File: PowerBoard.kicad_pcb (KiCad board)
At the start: 2 copper layers, 131 x 131 mm, 106 parts, among them IC1 LT1910ES8#PBF, IC2 LT1910ES8#PBF, IC3 LT1910ES8#PBF, IC4 LT1910ES8#PBF, J1 XT90, J10 DEAN_T, J11 DEAN_T, J12 DEAN_T, J13 DEAN_T, J14 DEAN_T, J15 DEAN_T, J16 XT60, J17 XT60, J18 XT60, J19 XT60, J2 DEAN_T, J20 XT60, J21 XT60, J22 XT30, J23 XT30, J24 XT30, J25 XT30, J26 XT30, J27 XT30, J28 XT90, J29 XT30, J3 XT60, J30 XT30, J31 XT30, J32 Conn_01x02, J4 XT30, J5 XT90, J6 XT90, J7 XT90, J8 XT90, J9 XT90, Q1 IRFS7437TRLPBF, Q2 IRFS7437TRLPBF, Q3 IRFS7437TRLPBF, Q5 IRFS7530-7PPBF, U1 Pico, U2 LM317_TO-220

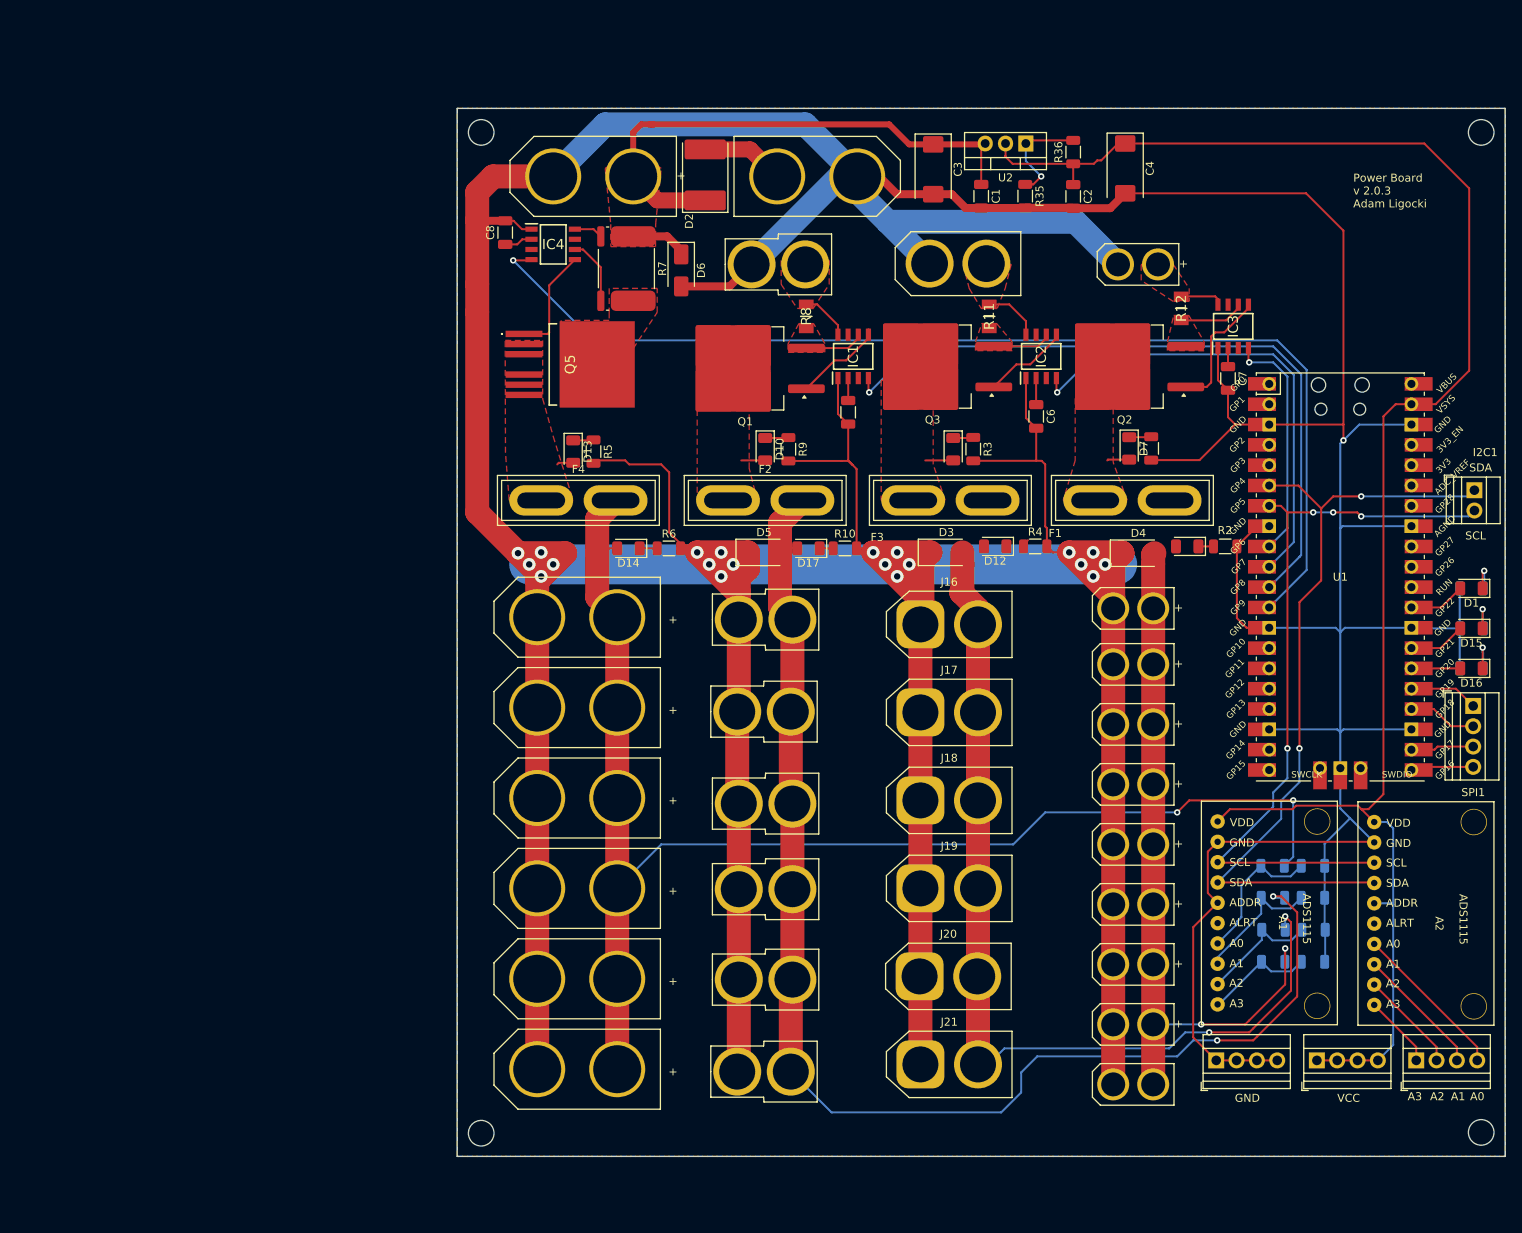
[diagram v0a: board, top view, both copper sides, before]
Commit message: Finish the design
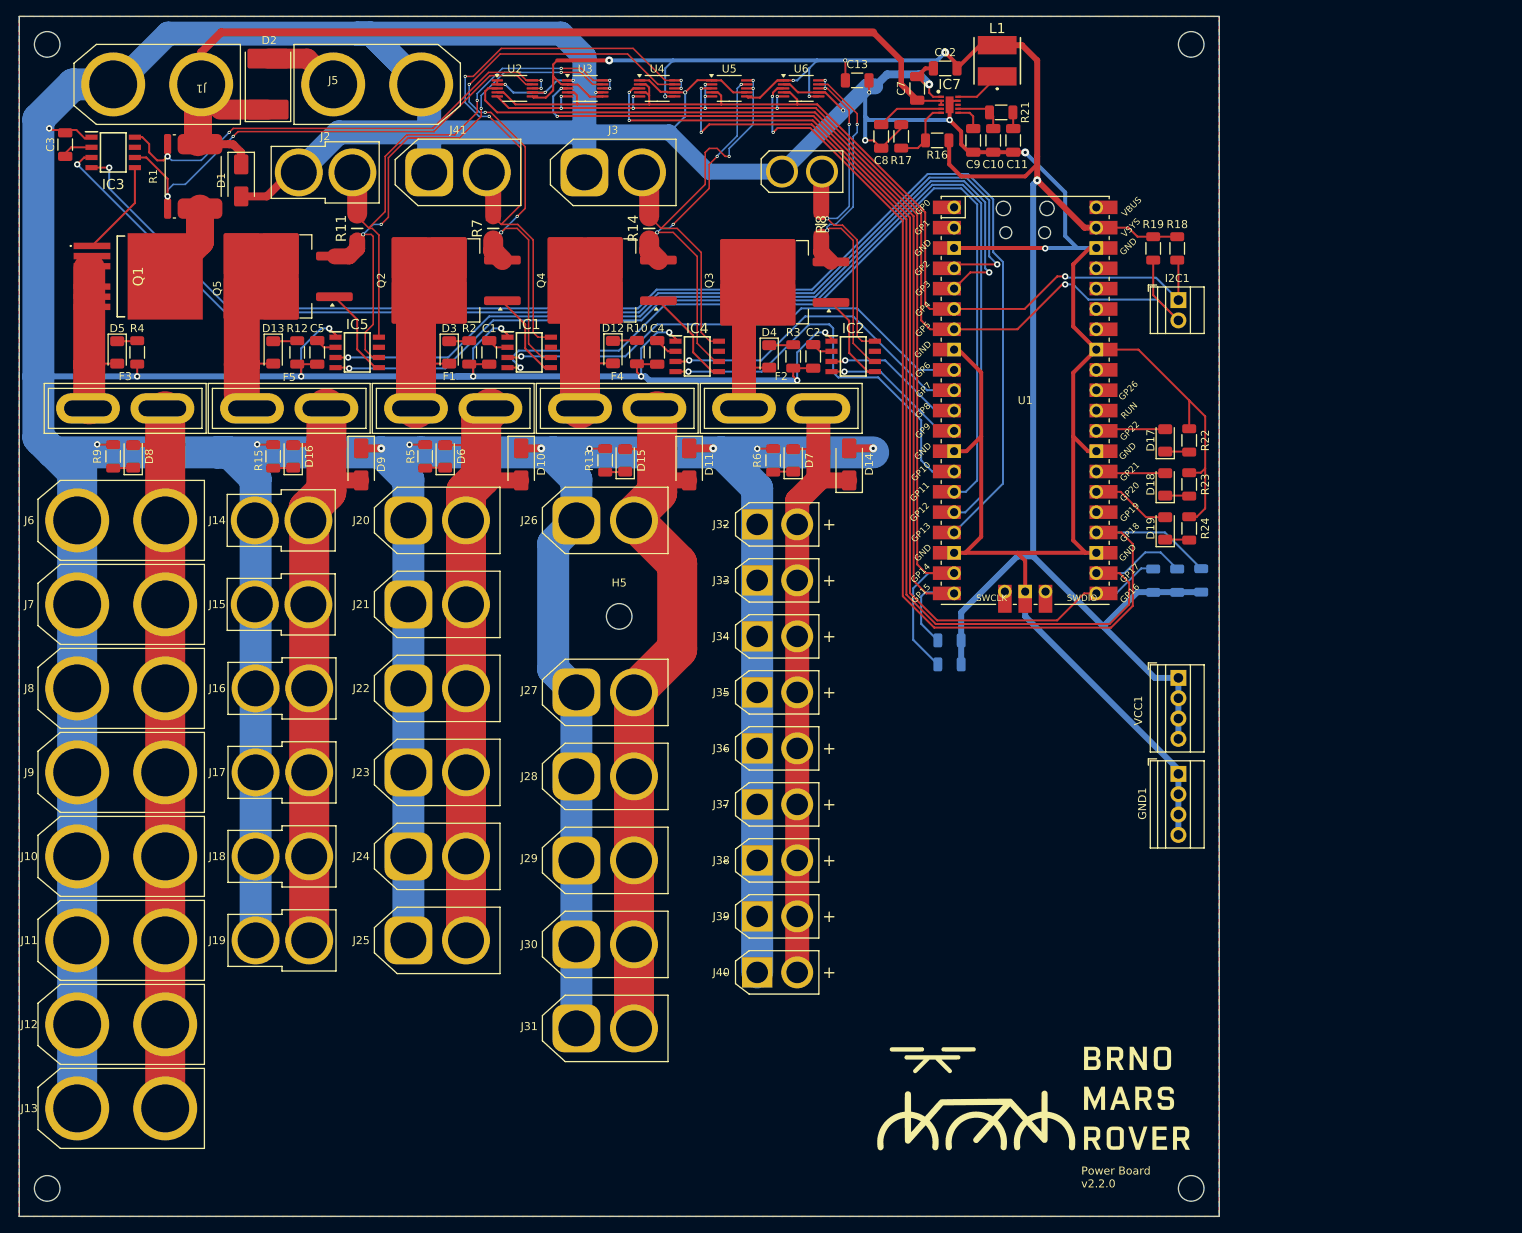
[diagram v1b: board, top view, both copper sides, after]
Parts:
- removed A1, A2: ADS1115_ADC_Module, my_footprint_lib:ADS1115
- removed ADC1, SPI1: Screw_Terminal_01x04, TerminalBlock:TerminalBlock_Xinya_XY308-2.54-4P_1x04_P2.54mm_Horizontal
- removed C6: 1u, Capacitor_SMD:C_1206_3216Metric
- removed R25, R32: 100k, Resistor_SMD:R_1206_3216Metric
- removed R30: 33k, Resistor_SMD:R_1206_3216Metric
- removed R31, R33, R39, R40: 10k, Resistor_SMD:R_1206_3216Metric
- removed R35: 680R, Resistor_SMD:R_1206_3216Metric
- removed R36: 220R, Resistor_SMD:R_1206_3216Metric
- added C10: 22pF, Capacitor_SMD:C_1206_3216Metric, F.Cu at (147.0, 33.5)
- added C11: 3300pF, Capacitor_SMD:C_1206_3216Metric, F.Cu at (149.5, 33.5)
- added C12: 10u, Capacitor_SMD:C_1206_3216Metric, F.Cu at (141.0, 24.5)
- added C13: 1u, Capacitor_SMD:C_1206_3216Metric, F.Cu at (130.0, 26.0)
- added C9: 5.5nF, Capacitor_SMD:C_1206_3216Metric, F.Cu at (144.5, 33.5)
- added D18: LED, Diode_SMD:D_1206_3216Metric, F.Cu at (168.5, 76.5)
- added D19: LED, Diode_SMD:D_1206_3216Metric, F.Cu at (168.5, 82.0)
- added D9: SMAJ30CA, Diode_SMD:D_SMA, F.Cu at (68.0, 74.0)
- added F5: Fuse, Fuse:Fuse_Blade_ATO_directSolder, F.Cu at (54.4, 67.0)
- added G***: LOGO, LOGO, F.Cu at (152.5, 153.5)
- added H5: MountingHole, MountingHole:MountingHole_3.2mm_M3, F.Cu at (100.2, 93.0)
- added IC5: LT1910ES8#PBF, SamacSys_Parts:SOIC127P599X175-8N, F.Cu at (67.5, 60.0)
- added IC7: MAX17541GATB+T, SamacSys_Parts:SON50P200X300X80-11N, F.Cu at (141.6, 29.1)
- added J33: XT30, Connector_AMASS:AMASS_XT30U-F_1x02_P5.0mm_Vertical, F.Cu at (117.5, 88.5)
- added J34: XT30, Connector_AMASS:AMASS_XT30U-F_1x02_P5.0mm_Vertical, F.Cu at (117.5, 95.5)
- added J35: XT30, Connector_AMASS:AMASS_XT30U-F_1x02_P5.0mm_Vertical, F.Cu at (117.5, 102.5)
- added J36: XT30, Connector_AMASS:AMASS_XT30U-F_1x02_P5.0mm_Vertical, F.Cu at (117.5, 109.5)
- added J37: XT30, Connector_AMASS:AMASS_XT30U-F_1x02_P5.0mm_Vertical, F.Cu at (117.5, 116.5)
- added J38: XT30, Connector_AMASS:AMASS_XT30U-F_1x02_P5.0mm_Vertical, F.Cu at (117.5, 123.5)
- added J39: XT30, Connector_AMASS:AMASS_XT30U-F_1x02_P5.0mm_Vertical, F.Cu at (117.5, 130.5)
- added J40: XT30, Connector_AMASS:AMASS_XT30U-F_1x02_P5.0mm_Vertical, F.Cu at (117.5, 137.5)
- added J41: XT60, Connector_AMASS:AMASS_XT60-F_1x02_P7.20mm_Vertical, F.Cu at (76.5, 37.5)
- added L1: 470M, SamacSys_Parts:SRR5828A2R6Y, F.Cu at (147.5, 23.6)
- added Q4: IRFS7437TRLPBF, Package_TO_SOT_SMD:TO-263-2, F.Cu at (97.5, 51.0)
- added R13: 6k8, Resistor_SMD:R_1206_3216Metric, F.Cu at (98.5, 73.5)
- added R14: 5m, SamacSys_Parts:RESC3216X89N, F.Cu at (104.0, 44.5)
- added R15: 6k8, Resistor_SMD:R_1206_3216Metric, F.Cu at (57.0, 73.0)
- added R16: 80k, Resistor_SMD:R_1206_3216Metric, F.Cu at (140.0, 33.5)
- added R17: 17.5k, Resistor_SMD:R_1206_3216Metric, F.Cu at (135.5, 33.0)
- added R18: 10k, Resistor_SMD:R_1206_3216Metric, F.Cu at (170.0, 47.0)
- added R19: 10k, Resistor_SMD:R_1206_3216Metric, F.Cu at (167.0, 47.0)
- added R20: 10k, Resistor_SMD:R_1206_3216Metric, B.Cu at (141.5, 99.0)
- added R21: 21.5k, Resistor_SMD:R_1206_3216Metric, F.Cu at (148.0, 30.0)
- added R22: 10k, Resistor_SMD:R_1206_3216Metric, F.Cu at (171.5, 71.0)
- added R23: 10k, Resistor_SMD:R_1206_3216Metric, F.Cu at (171.5, 76.5)
- added R24: 10k, Resistor_SMD:R_1206_3216Metric, F.Cu at (171.5, 82.0)
- added U3: INA238, Package_SO:VSSOP-10_3x3mm_P0.5mm, F.Cu at (96.0, 27.0)
- added U4: INA238, Package_SO:VSSOP-10_3x3mm_P0.5mm, F.Cu at (105.0, 27.0)
- added U5: INA238, Package_SO:VSSOP-10_3x3mm_P0.5mm, F.Cu at (114.0, 27.0)
- added U6: INA238, Package_SO:VSSOP-10_3x3mm_P0.5mm, F.Cu at (123.0, 27.0)
- C3, C4: value 10u -> 1u; footprint Capacitor_Tantalum_SMD:CP_EIA-7343-15_Kemet-W -> Capacitor_SMD:C_1206_3216Metric
- D1: value LED -> SMAJ48A; footprint Diode_SMD:D_1206_3216Metric -> Diode_SMD:D_SMA
- D10: value LED -> SMAJ30CA; footprint Diode_SMD:D_1206_3216Metric -> Diode_SMD:D_SMA
- D11: value LED -> SMAJ15CA; footprint Diode_SMD:D_1206_3216Metric -> Diode_SMD:D_SMA
- D14: value LED -> SMAJ6.5CA; footprint Diode_SMD:D_1206_3216Metric -> Diode_SMD:D_SMA
- D3: value SMAJ15CA -> LED; footprint Diode_SMD:D_SMA -> Diode_SMD:D_1206_3216Metric
- D4: value SMAJ6.5CA -> LED; footprint Diode_SMD:D_SMA -> Diode_SMD:D_1206_3216Metric
- D5: value SMAJ30CA -> LED; footprint Diode_SMD:D_SMA -> Diode_SMD:D_1206_3216Metric
- D6: value SMAJ48A -> LED; footprint Diode_SMD:D_SMA -> Diode_SMD:D_1206_3216Metric
- J1, J6, J7, J8, J9: footprint my_footprint_lib:XT90 -> SamacSys_Parts:XT90
- J10, J11, J12, J13: value DEAN_T -> XT90; footprint my_footprint_lib:DEAN_T -> SamacSys_Parts:XT90
- J14, J15, J2: footprint my_footprint_lib:DEAN_T -> SamacSys_Parts:DEANS-T
- J16, J17, J18, J19: value XT60 -> DEAN_T; footprint Connector_AMASS:AMASS_XT60-F_1x02_P7.20mm_Vertical -> SamacSys_Parts:DEANS-T
- J22, J23, J24, J25, J26, J27, J29, J30, J31: value XT30 -> XT60; footprint my_footprint_lib:XT30 -> Connector_AMASS:AMASS_XT60-F_1x02_P7.20mm_Vertical
- J28: value XT90 -> XT60; footprint my_footprint_lib:XT90 -> Connector_AMASS:AMASS_XT60-F_1x02_P7.20mm_Vertical
- J3: footprint my_footprint_lib:XT60 -> Connector_AMASS:AMASS_XT60-F_1x02_P7.20mm_Vertical
- J32: value Conn_01x02 -> XT30; footprint my_footprint_lib:XT90 -> Connector_AMASS:AMASS_XT30U-F_1x02_P5.0mm_Vertical
- J5: value XT90 -> Conn_01x02; footprint my_footprint_lib:XT90 -> SamacSys_Parts:XT90
- Q1: value IRFS7437TRLPBF -> IRFS7530TRL7PP; footprint Package_TO_SOT_SMD:TO-263-2 -> SamacSys_Parts:IRFS7530TRL7PP
- Q5: value IRFS7530-7PPBF -> IRFS7437TRLPBF; footprint SamacSys_Parts:IRFS41157PPBF -> Package_TO_SOT_SMD:TO-263-2
- R1: value 6k8 -> 4m; footprint Resistor_SMD:R_1206_3216Metric -> Resistor_SMD:R_Shunt_Isabellenhuette_BVR4026
- R11: value 5m -> 1m
- R12: value 5m -> 6k8; footprint SamacSys_Parts:RESC3216X89N -> Resistor_SMD:R_1206_3216Metric
- R27, R29: value 100k -> 10k
- R7: value 4m -> 5m; footprint Resistor_SMD:R_Shunt_Isabellenhuette_BVR4026 -> SamacSys_Parts:RESC3216X89N
- R8: value 1m -> 5m
- U2: value LM317_TO-220 -> INA238; footprint Package_TO_SOT_THT:TO-220-3_Vertical -> Package_SO:VSSOP-10_3x3mm_P0.5mm
- moved D1 162.0 mm to (53.0, 38.5), turned to -90 degrees
- moved D16 149.6 mm to (59.5, 73.0), turned to 90 degrees
- moved IC3 141.7 mm to (37.0, 35.0), turned to 0 degrees
- moved D8 132.2 mm to (39.5, 73.0), turned to 90 degrees
- moved R1 124.5 mm to (47.0, 38.0)
- moved R4 114.8 mm to (40.0, 60.0), turned to -90 degrees
- moved R12 110.6 mm to (60.0, 60.0)
- moved C3 108.5 mm to (31.0, 34.0), turned to 90 degrees
- moved D15 107.8 mm to (101.0, 73.5), turned to 90 degrees
- moved F3 103.8 mm to (33.9, 67.0)
- moved R2 97.6 mm to (81.5, 60.0), turned to -90 degrees
- moved J15 91.4 mm to (58.0, 91.5)
- moved J14 90.9 mm to (58.0, 81.0)
- moved J25 87.2 mm to (73.9, 133.5)
- moved J24 86.6 mm to (73.9, 123.0)
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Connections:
- C1 pad 1: +42V -> Net-(IC1-TIMER)
- C2 pad 1: VCC -> Net-(IC2-TIMER)
- C3 pad 1: +42V -> Net-(IC3-TIMER)
- C4 pad 1: VCC -> Net-(IC4-TIMER)
- C5 pad 1: Net-(IC1-TIMER) -> Net-(IC5-TIMER)
- C7 pad 1: Net-(IC3-TIMER) -> +42V
- C8 pad 1: Net-(IC4-TIMER) -> Net-(IC7-VCC)
- D1 pad 1: Net-(D1-K) -> +42V
- D1 pad 2: Net-(D1-A) -> GND
- D10 pad 1: Net-(D10-K) -> GND
- D10 pad 2: Net-(D10-A) -> 15V_2
- D11 pad 1: Net-(D11-K) -> GND
- D11 pad 2: Net-(D11-A) -> 12V_2
- D12 pad 2: 12V_2 -> Net-(D12-A)
- D14 pad 1: Net-(D14-K) -> 5V_2
- D14 pad 2: 42V_2 -> GND
- D15 pad 2: Net-(D15-A) -> 12V_2
- D16 pad 2: Net-(D16-A) -> 24V_2
- D17 pad 2: 24V_2 -> Net-(D17-A)
- D3 pad 1: GND -> Net-(D3-K)
- D3 pad 2: 12V_2 -> Net-(D3-A)
- D4 pad 1: GND -> Net-(D4-K)
- D4 pad 2: 5V_2 -> Net-(D4-A)
- D5 pad 1: GND -> Net-(D5-K)
- D5 pad 2: 24V_2 -> Net-(D5-A)
- D6 pad 1: +42V -> Net-(D6-K)
- D6 pad 2: GND -> 15V_2
- D7 pad 2: Net-(D7-A) -> 5V_2
- D8 pad 2: 5V_2 -> 42V_2
- F1 pad 1: Net-(D7-A) -> Net-(D3-A)
- F1 pad 2: 5V_2 -> 15V_2
- F2 pad 1: Net-(D10-A) -> Net-(D4-A)
- F2 pad 2: 24V_2 -> 5V_2
- F3 pad 1: Net-(D11-A) -> Net-(D5-A)
- F3 pad 2: 12V_2 -> 42V_2
- F4 pad 1: Net-(D13-A) -> Net-(D12-A)
- F4 pad 2: 42V_2 -> 12V_2
- IC1 pad 3: unconnected-(IC1-~{FAULT}-Pad3) -> FAULT_15V
- IC1 pad 4: EN_24V -> EN_15V
- IC1 pad 6: Net-(IC1-SENSE) -> CURR_3-
- IC1 pad 8: +24V -> CURR_3+
- IC2 pad 3: unconnected-(IC2-~{FAULT}-Pad3) -> FAULT_5V
- IC2 pad 4: EN_12V -> EN_5V
- IC2 pad 6: Net-(IC2-SENSE) -> CURR_5-
- IC2 pad 8: +12V -> CURR_5+
- IC3 pad 3: unconnected-(IC3-~{FAULT}-Pad3) -> FAULT_42V
- IC3 pad 4: EN_5V -> EN_42V
- IC3 pad 6: Net-(IC3-SENSE) -> CURR_1-
- IC3 pad 8: +5V -> CURR_1+
- IC4 pad 3: unconnected-(IC4-~{FAULT}-Pad3) -> FAULT_12V
- IC4 pad 4: EN_42V -> EN_12V
- IC4 pad 6: Net-(IC4-SENSE) -> CURR_4-
- IC4 pad 8: Net-(IC4-V+) -> CURR_4+
- J10 pad 1: 24V_2 -> 42V_2
- J11 pad 1: 24V_2 -> 42V_2
- J12 pad 1: 24V_2 -> 42V_2
- J13 pad 1: 24V_2 -> 42V_2
- J14 pad 1: 24V_2 -> GND
- J14 pad 2: GND -> 24V_2
- J15 pad 1: 24V_2 -> GND
- J15 pad 2: GND -> 24V_2
- J16 pad 2: 12V_2 -> 24V_2
- J17 pad 2: 12V_2 -> 24V_2
- J18 pad 2: 12V_2 -> 24V_2
- J19 pad 2: 12V_2 -> 24V_2
- J2 pad 1: +24V -> GND
- J2 pad 2: GND -> CURR_2+
- J20 pad 2: 12V_2 -> 15V_2
- J21 pad 2: 12V_2 -> 15V_2
- J22 pad 1: 5V_2 -> GND
- J22 pad 2: GND -> 15V_2
- J23 pad 1: 5V_2 -> GND
- J23 pad 2: GND -> 15V_2
- J24 pad 1: 5V_2 -> GND
- J24 pad 2: GND -> 15V_2
- J25 pad 1: 5V_2 -> GND
- J25 pad 2: GND -> 15V_2
- J26 pad 1: 5V_2 -> GND
- J26 pad 2: GND -> 12V_2
- J27 pad 1: 5V_2 -> GND
- J27 pad 2: GND -> 12V_2
- J28 pad 1: 42V_2 -> GND
- J28 pad 2: GND -> 12V_2
- J29 pad 1: 5V_2 -> GND
- J29 pad 2: GND -> 12V_2
- J3 pad 1: +12V -> GND
- J3 pad 2: GND -> CURR_4+
- J30 pad 1: 5V_2 -> GND
- J30 pad 2: GND -> 12V_2
- J31 pad 1: 5V_2 -> GND
- J31 pad 2: GND -> 12V_2
- J32 pad 1: Net-(D2-A) -> GND
- J32 pad 2: GND -> 5V_2
- J4 pad 1: +5V -> CURR_5+
- J5 pad 1: 42V_2 -> Net-(D2-A)
- Q1 pad 1: Net-(IC1-GATE) -> Net-(IC3-GATE)
- Q1 pad 2: Net-(D10-A) -> Net-(D5-A)
- Q1 pad 3: Net-(IC1-SENSE) -> Net-(D5-A)
- Q2 pad 1: Net-(IC3-GATE) -> Net-(IC1-GATE)
- Q2 pad 2: Net-(D7-A) -> Net-(D3-A)
- Q2 pad 3: Net-(IC3-SENSE) -> CURR_3-
- Q3 pad 2: Net-(D11-A) -> Net-(D4-A)
- Q3 pad 3: Net-(IC2-SENSE) -> CURR_5-
- Q5 pad 1: Net-(IC4-GATE) -> Net-(IC5-GATE)
- Q5 pad 3: Net-(D13-A) -> CURR_2-
- R1 pad 1: Net-(D7-K) -> +42V
- R1 pad 2: GND -> CURR_1+
- R10 pad 1: Net-(D17-K) -> Net-(D12-K)
- R11 pad 1: +12V -> CURR_2-
- R11 pad 2: Net-(IC2-SENSE) -> CURR_2+
- R12 pad 1: +5V -> Net-(D13-K)
- R12 pad 2: Net-(IC3-SENSE) -> GND
- R2 pad 1: Net-(D8-K) -> Net-(D3-K)
- R26 pad 1: Net-(A1-A0) -> VCC
- R26 pad 2: GND -> ALERT_2
- R27 pad 1: 24V_2 -> VCC
- R27 pad 2: Net-(A1-A1) -> ALERT_3
- R28 pad 1: Net-(A1-A1) -> VCC
- R28 pad 2: GND -> ALERT_4
- R29 pad 1: 12V_2 -> VCC
- R29 pad 2: Net-(A1-A2) -> ALERT_5
- R3 pad 1: Net-(D11-K) -> Net-(D4-K)
- R4 pad 1: Net-(D12-K) -> Net-(D5-K)
- R5 pad 1: Net-(D13-K) -> Net-(D6-K)
- R6 pad 1: Net-(D14-K) -> Net-(D7-K)
- R7 pad 1: +42V -> CURR_3+
- R7 pad 2: Net-(IC4-V+) -> CURR_3-
- R8 pad 1: Net-(IC1-SENSE) -> CURR_5+
- R8 pad 2: +24V -> CURR_5-
- R9 pad 1: Net-(D10-K) -> Net-(D8-K)
- U1 pad 10: EN_12V -> FAULT_12V
- U1 pad 11: EN_24V -> FAULT_5V
- U1 pad 12: EN_42V -> EN_5V
- U1 pad 14: unconnected-(U1-GPIO10-Pad14) -> EN_12V
- U1 pad 15: unconnected-(U1-GPIO11-Pad15) -> EN_15V
- U1 pad 16: unconnected-(U1-GPIO12-Pad16)_1 -> EN_24V
- U1 pad 17: unconnected-(U1-GPIO13-Pad17)_1 -> EN_42V
- U1 pad 19: unconnected-(U1-GPIO14-Pad19) -> ALERT_1
- U1 pad 20: unconnected-(U1-GPIO15-Pad20)_1 -> ALERT_2
- U1 pad 21: Net-(SPI1-Pin_4) -> ALERT_3
- U1 pad 22: Net-(SPI1-Pin_3) -> ALERT_4
- U1 pad 24: Net-(SPI1-Pin_2) -> ALERT_5
- U1 pad 25: Net-(SPI1-Pin_1) -> unconnected-(U1-GPIO19-Pad25)
- U1 pad 26: Net-(D16-A) -> Net-(D19-A)
- U1 pad 27: Net-(D15-A) -> Net-(D18-A)
- U1 pad 29: Net-(D1-A) -> Net-(D17-A)
- U1 pad 4: unconnected-(U1-GPIO2-Pad4) -> FAULT_42V
- U1 pad 5: unconnected-(U1-GPIO3-Pad5) -> FAULT_24V
- U1 pad 9: EN_5V -> FAULT_15V
- U2 pad 1: Net-(U2-ADJ) -> GND
- U2 pad 2: VCC -> GND
- U2 pad 3: +42V -> ALERT_1
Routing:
- net GND: track 1017.3 -> 1201.6 mm, vias 21 -> 31
- net FAULT_42V: track 0.00 -> 146.0 mm, vias 0 -> 2
- net ALERT_4: track 0.00 -> 134.5 mm, vias 0 -> 2
- net ALERT_5: track 0.00 -> 134.1 mm, vias 0 -> 2
- net ALERT_1: track 0.00 -> 128.2 mm
- net ALERT_3: track 0.00 -> 126.6 mm, vias 0 -> 2
- net ALERT_2: track 0.00 -> 116.7 mm, vias 0 -> 2
- net EN_15V: track 0.00 -> 108.9 mm, vias 0 -> 1
- net FAULT_24V: track 0.00 -> 105.6 mm, vias 0 -> 2
- net 24V_2: track 164.5 -> 76.6 mm, vias 2 -> 0
- net 42V_2: track 174.0 -> 91.7 mm, vias 2 -> 0
- net CURR_3+: track 0.00 -> 79.6 mm, vias 0 -> 4
- net CURR_3-: track 0.00 -> 77.3 mm, vias 0 -> 4
- net 15V_2: track 0.00 -> 77.0 mm
- net CURR_2+: track 0.00 -> 68.8 mm, vias 0 -> 4
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- removed copper zone on F.Cu, net +12V
- removed copper zone on F.Cu, net +24V
- removed copper zone on F.Cu, net +42V
- removed copper zone on F.Cu, net +5V
- removed copper zone on F.Cu, net Net-(D10-A)
- removed copper zone on F.Cu, net Net-(D11-A)
- removed copper zone on F.Cu, net Net-(D13-A)
- removed copper zone on F.Cu, net Net-(D7-A)
- removed copper zone on F.Cu, net Net-(IC1-SENSE)
- removed copper zone on F.Cu, net Net-(IC2-SENSE)
- removed copper zone on F.Cu, net Net-(IC3-SENSE)
- removed copper zone on F.Cu, net Net-(Q5-D)
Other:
- board size 131 x 131 mm -> 150 x 150 mm
- board text added: "Power Board v2.2.0"
- board text removed: "A0"
- board text removed: "A1"
- board text removed: "A2"
- board text removed: "A3"
- board text removed: "GND"
- board text removed: "Power Board v 2.0.3 Adam Ligocki"
- board text removed: "SCL"
- board text removed: "SDA"
- board text removed: "VCC"
